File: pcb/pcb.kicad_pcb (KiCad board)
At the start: 2 copper layers, 17 parts, among them U1 L293D

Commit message: added l293d en / PWM pin connection
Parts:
- added REF**: ., Connector_Wire:SolderWirePad_1x01_Drill0.8mm, F.Cu at (104.1, 69.8)
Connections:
- U1 pad 1: Net-(A1-Pad22) -> Net-(A1-Pad8)
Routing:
- net Net-(A1-Pad22): track 9.20 -> 0.00 mm
- net Net-(A1-Pad8): track 3.81 -> 6.35 mm

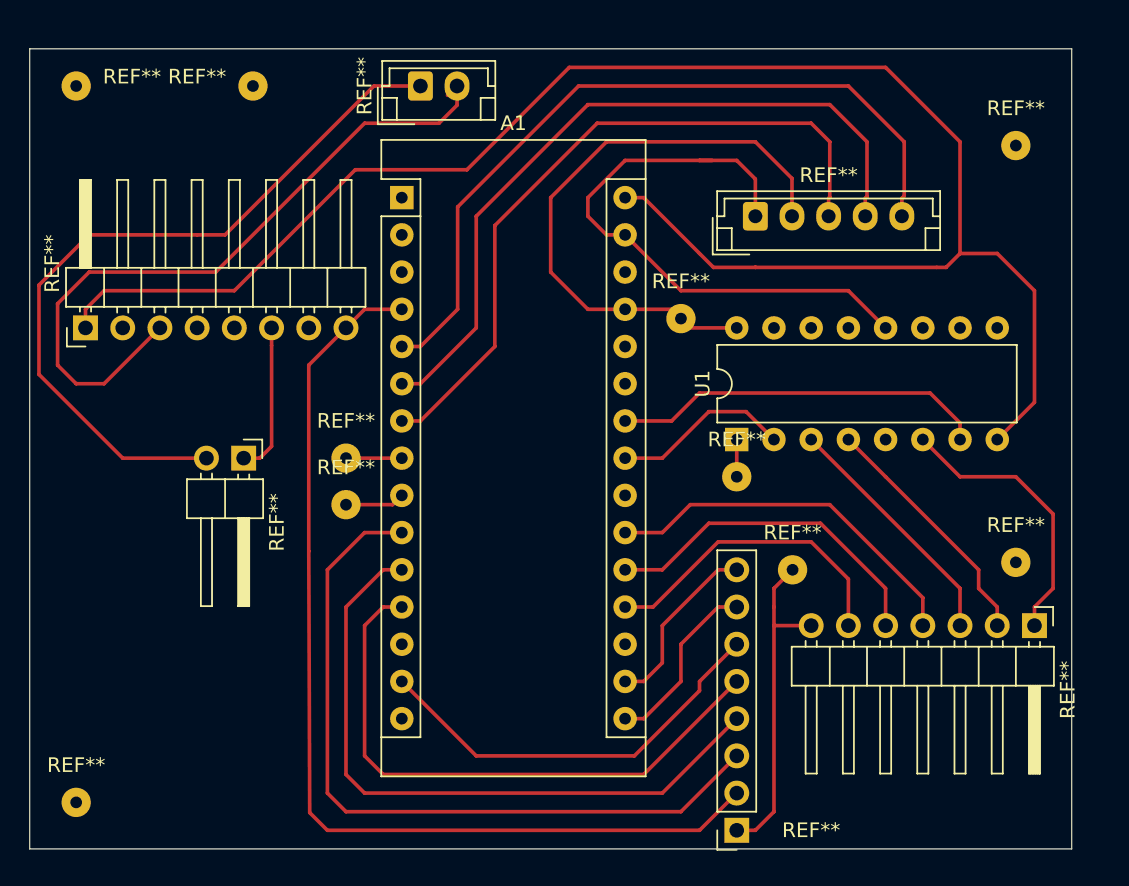
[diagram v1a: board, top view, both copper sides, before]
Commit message: general update
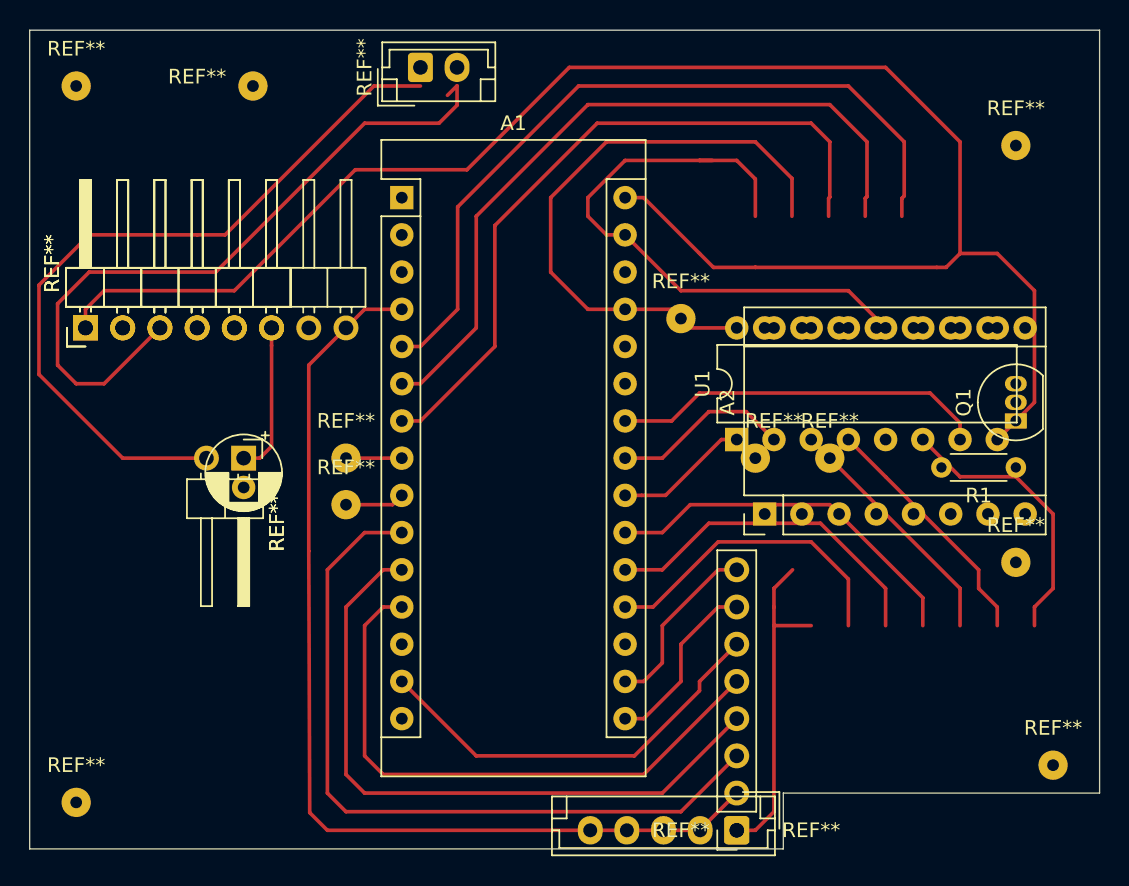
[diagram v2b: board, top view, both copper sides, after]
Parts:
- removed the REF** at (104.1, 69.8)
- removed the REF** at (70.5, 68.6)
- removed the REF** at (104.1, 94.0)
- removed the REF** at (59.7, 59.7)
- removed the REF** at (105.4, 52.1)
- removed the REF** at (108.0, 76.2)
- removed the REF** at (124.5, 80.0)
- added A2: A4988, Module:Pololu_Breakout-16_15.2x20.3mm, F.Cu at (106.0, 72.4)
- added Q1: 2N3906, Package_TO_SOT_THT:TO-92_Inline, F.Cu at (123.2, 66.0)
- added R1: R, Resistor_THT:R_Axial_DIN0204_L3.6mm_D1.6mm_P5.08mm_Horizontal, F.Cu at (123.2, 69.2)
- added REF**: pad, Connector_Wire:SolderWirePad_1x01_Drill0.8mm, F.Cu at (110.5, 68.6)
- added REF**: pad, Connector_Wire:SolderWirePad_1x01_Drill0.8mm, F.Cu at (105.4, 68.6)
- added REF** (x2): PinHeader_1x02_P2.54mm_Horizontal, Connector_PinHeader_2.54mm:PinHeader_1x02_P2.54mm_Horizontal, F.Cu at (70.5, 68.6)
- added REF** (x2): PinSocket_1x08_P2.54mm_Vertical, Connector_PinSocket_2.54mm:PinSocket_1x08_P2.54mm_Vertical, F.Cu at (104.1, 94.0)
- added REF**: PinHeader_1x08_P2.54mm_Horizontal, Connector_PinHeader_2.54mm:PinHeader_1x08_P2.54mm_Horizontal, F.Cu at (59.7, 59.7)
- added REF**: ., Connector_Wire:SolderWirePad_1x01_Drill0.8mm, F.Cu at (125.7, 89.5)
- added REF**: PinHeader_1x07_P2.54mm_Horizontal, Connector_PinHeader_2.54mm:PinHeader_1x08_P2.54mm_Horizontal, F.Cu at (59.7, 59.7)
- moved REF** 1.27 mm to (82.5, 41.9)
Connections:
- REF** pad 1: Net-(A1-Pad9) -> (no net)
- REF** pad 1: (no net) -> Net-(A1-Pad21)
- REF** pad 1: (no net) -> end_signal
- REF** pad 1: Net-(A1-Pad8) -> (no net)
- U1 pad 1: Net-(A1-Pad8) -> Net-(A1-Pad22)
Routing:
- net Net-(A1-Pad22): track 0.00 -> 9.20 mm
- net Net-(A1-Pad8): track 6.35 -> 3.81 mm
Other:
- board size 71.1 x 54.6 mm -> 73 x 55.9 mm
